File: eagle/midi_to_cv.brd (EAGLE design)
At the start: 100 x 80 mm, 71 parts, among them IC1 TL084P, IC4 TL072P, U1 ATMEGA328P_PDIP, U4 4584N

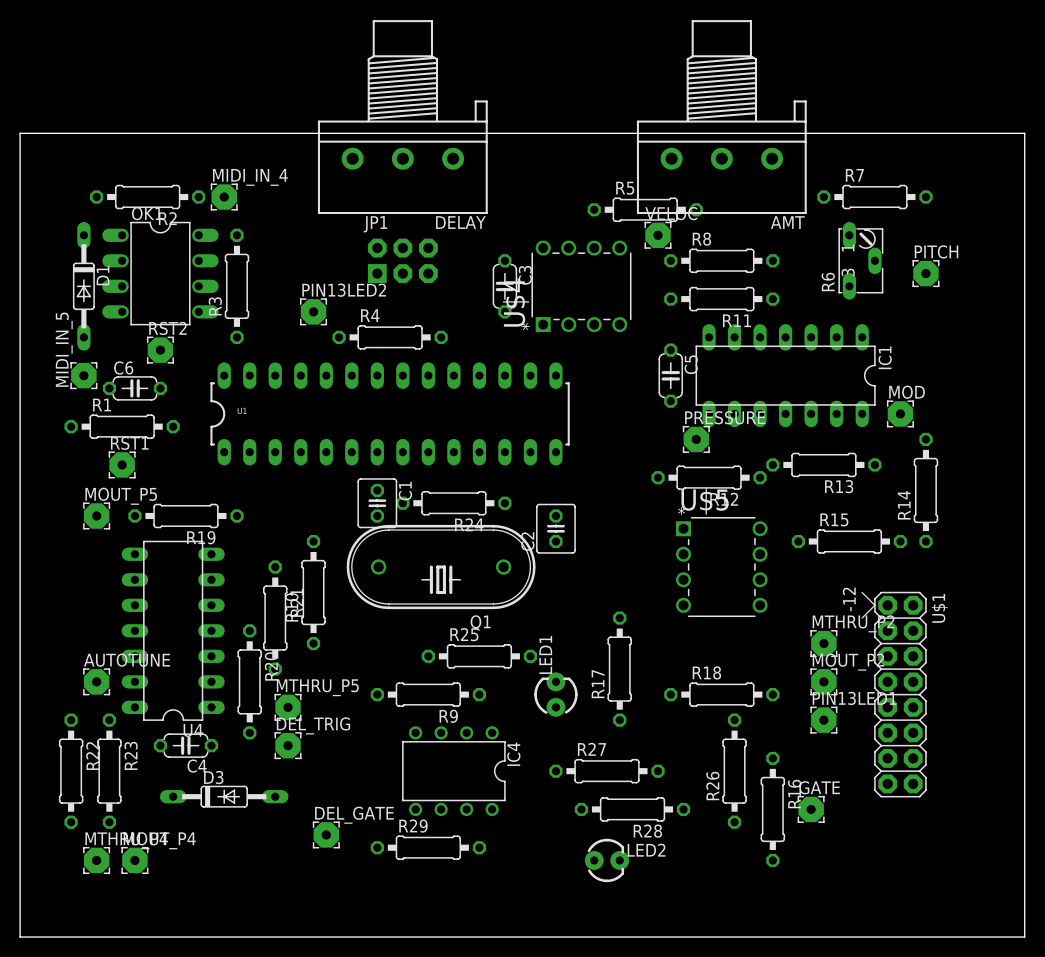
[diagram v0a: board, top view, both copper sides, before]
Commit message: ready to cut layout
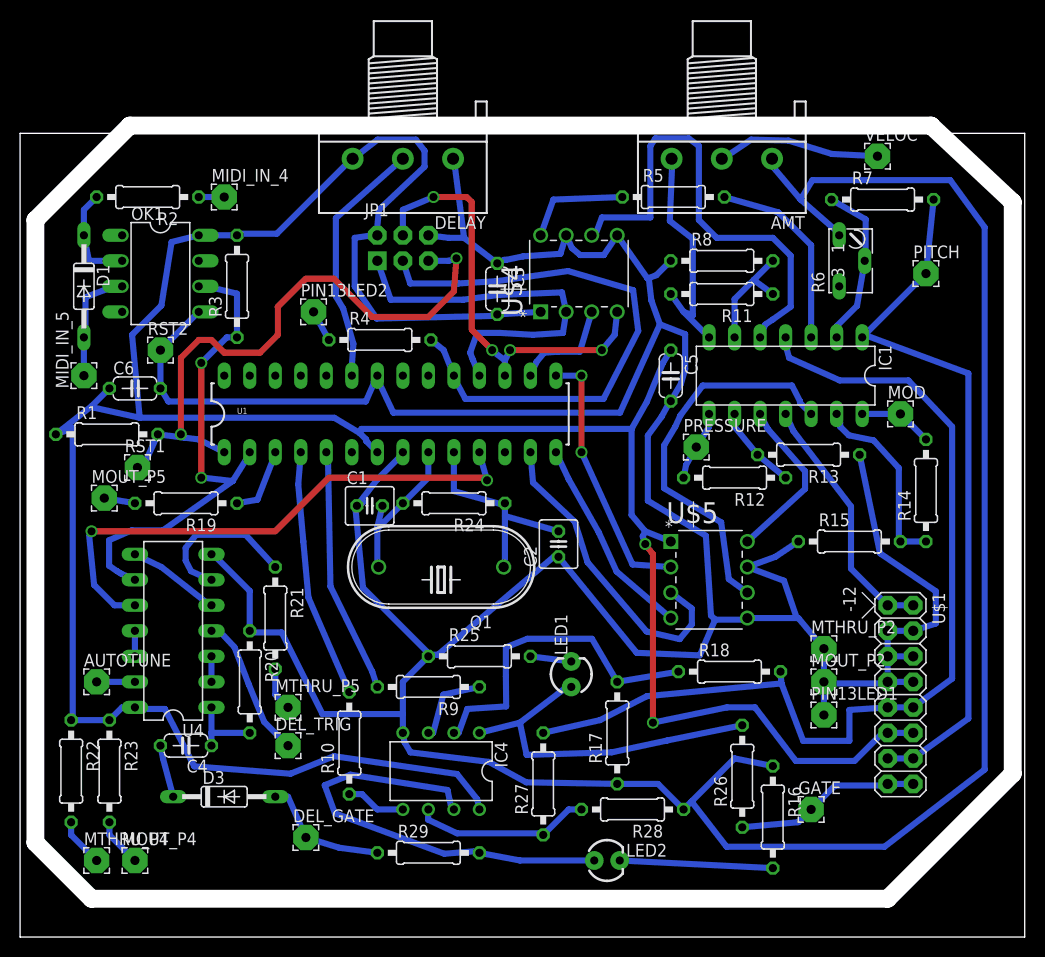
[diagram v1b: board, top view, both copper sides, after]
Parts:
- R18, R27: value 20k -> 47k
- moved VELOC 23.2 mm to (85.3, 77.7)
- moved R10 15.4 mm to (32.8, 19.3)
- moved R27 6.48 mm to (52.1, 15.2), turned to 90 degrees
- moved R17 6.36 mm to (59.4, 20.3)
- moved R5 3.07 mm to (65.0, 73.7)
- moved R12 2.54 mm to (71.1, 45.7)
- moved LED1 2.54 mm to (54.9, 26.2)
- moved R18 2.41 mm to (70.6, 26.4)
- moved DEL_GATE 2.05 mm to (28.4, 9.91)
- moved MOUT_P5 1.93 mm to (8.38, 43.7)
- moved R13 1.83 mm to (78.5, 48.0)
- moved U$5 1.80 mm to (72.4, 31.8)
- moved R1 1.70 mm to (8.64, 50.0)
- moved C2 1.55 mm to (53.6, 39.1)
- moved RST1 1.55 mm to (11.7, 46.7)
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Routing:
- net GND: track 0.00 -> 489.9 mm
- net +5V: track 0.00 -> 300.3 mm, vias 0 -> 2
- net +12V: track 0.00 -> 96.5 mm
- net N$9: track 0.00 -> 71.3 mm
- net N$43: track 0.00 -> 60.9 mm, vias 0 -> 2
- net N$10: track 0.00 -> 57.3 mm
- net N$38: track 0.00 -> 55.0 mm, vias 0 -> 2
- net N$30: track 0.00 -> 50.3 mm, vias 0 -> 2
- net N$14: track 0.00 -> 47.5 mm
- net N$53: track 0.00 -> 44.4 mm
- net N$26: track 0.00 -> 43.4 mm, vias 0 -> 4
- net N$45: track 0.00 -> 38.4 mm
- net N$24: track 0.00 -> 38.3 mm
- net N$16: track 0.00 -> 36.4 mm
- net N$15: track 0.00 -> 32.6 mm
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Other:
- board size 100 x 80 mm -> 100 x 80.8 mm
